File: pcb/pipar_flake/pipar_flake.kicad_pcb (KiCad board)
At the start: 2 copper layers, 74.1 x 55 mm, 22 parts, among them SW2 SW_Wuerth_450301014042, U2 nice_nano

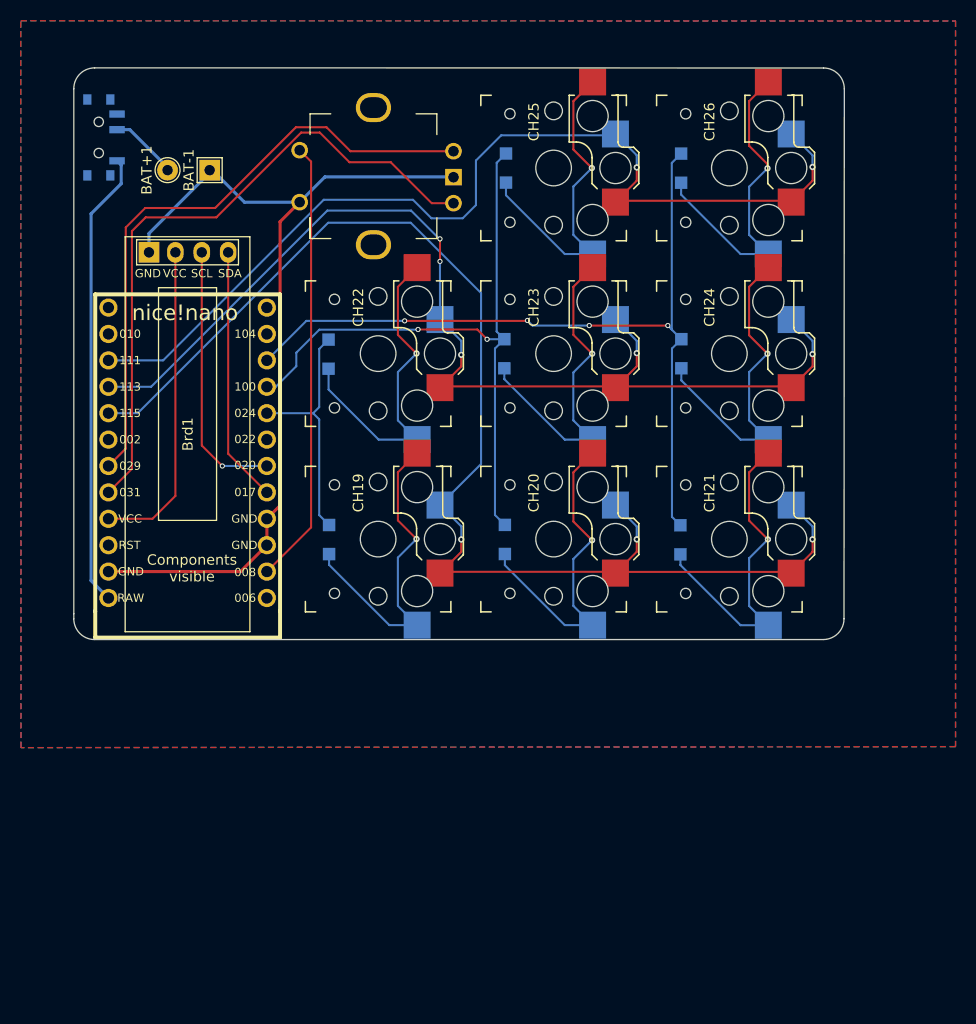
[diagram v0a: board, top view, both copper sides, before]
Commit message: Reworks Pipar Flake to add LEDs and a bigger place for battery
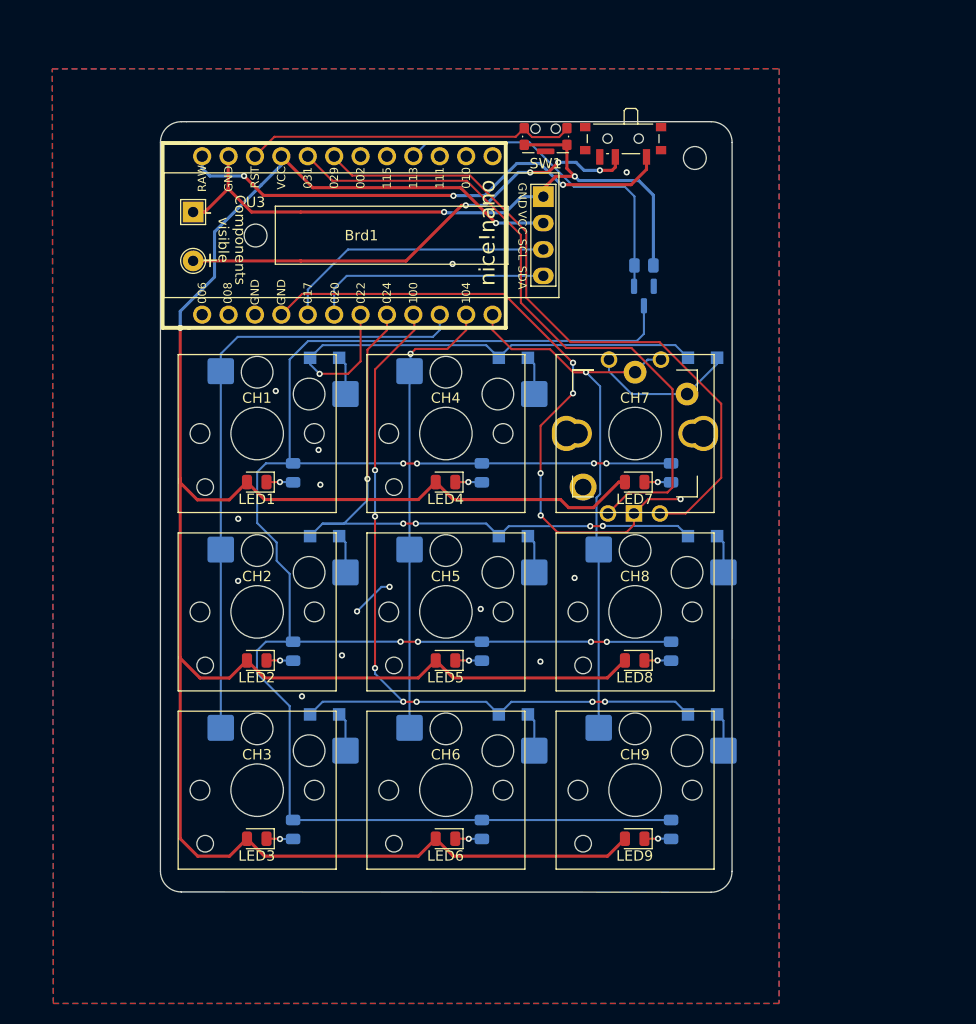
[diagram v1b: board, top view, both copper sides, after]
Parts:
- removed CH19, CH20, CH21, CH22, CH23, CH24, CH25, CH26: KSwitch, keyswitches:Kailh_socket_PG1350_reversible
- removed CH28: RotaryEncoder_Switch, Rotary_Encoder:RotaryEncoder_Bourns_Vertical_PEL11L-4xxxF-Sxxxx_1
- removed D19, D20, D21, D22, D23, D24, D25, D26: D, Diode_SMD:Nexperia_CFP3_SOD-123W
- added CH1: KSwitch, yes:SW_Hotswap_Kailh_Choc_V1V2_LED_1.00u, F.Cu at (32.8, 49.8)
- added CH10: RotaryEncoder_Switch, Rotary_Encoder:RotaryEncoder_Bourns_Vertical_PEL11L-4xxxF-Sxxxx_1, F.Cu at (69.1, 49.7)
- added CH2: KSwitch, yes:SW_Hotswap_Kailh_Choc_V1V2_LED_1.00u, F.Cu at (32.8, 66.9)
- added CH3: KSwitch, yes:SW_Hotswap_Kailh_Choc_V1V2_LED_1.00u, F.Cu at (32.8, 84.1)
- added CH4: KSwitch, yes:SW_Hotswap_Kailh_Choc_V1V2_LED_1.00u, F.Cu at (51.0, 49.8)
- added CH5: KSwitch, yes:SW_Hotswap_Kailh_Choc_V1V2_LED_1.00u, F.Cu at (51.0, 66.9)
- added CH6: KSwitch, yes:SW_Hotswap_Kailh_Choc_V1V2_LED_1.00u, F.Cu at (51.0, 84.1)
- added CH7: KSwitch, PCM_Switch_Keyboard_Kailh:SW_Kailh_Choc_V1V2_1.00u, F.Cu at (69.2, 49.8)
- added CH8: KSwitch, yes:SW_Hotswap_Kailh_Choc_V1V2_LED_1.00u, F.Cu at (69.2, 66.9)
- added CH9: KSwitch, yes:SW_Hotswap_Kailh_Choc_V1V2_LED_1.00u, F.Cu at (69.2, 84.1)
- added D1: D, Diode_SMD:Nexperia_CFP3_SOD-123W, B.Cu at (39.3, 42.5)
- added D2: D, Diode_SMD:Nexperia_CFP3_SOD-123W, B.Cu at (39.3, 59.7)
- added D3: D, Diode_SMD:Nexperia_CFP3_SOD-123W, B.Cu at (39.3, 76.8)
- added D4: D, Diode_SMD:Nexperia_CFP3_SOD-123W, B.Cu at (57.5, 42.5)
- added D5: D, Diode_SMD:Nexperia_CFP3_SOD-123W, B.Cu at (57.5, 59.7)
- added D6: D, Diode_SMD:Nexperia_CFP3_SOD-123W, B.Cu at (57.5, 76.8)
- added D7: D, Diode_SMD:Nexperia_CFP3_SOD-123W, B.Cu at (75.7, 42.5)
- added D8: D, Diode_SMD:Nexperia_CFP3_SOD-123W, B.Cu at (75.7, 59.6)
- added D9: D, Diode_SMD:Nexperia_CFP3_SOD-123W, B.Cu at (75.7, 76.8)
- added LED1: ~, LED_SMD:LED_0805_2012Metric, F.Cu at (32.8, 54.5)
- added LED2: ~, LED_SMD:LED_0805_2012Metric, F.Cu at (32.8, 71.6)
- added LED3: ~, LED_SMD:LED_0805_2012Metric, F.Cu at (32.8, 88.8)
- added LED4: ~, LED_SMD:LED_0805_2012Metric, F.Cu at (50.9, 54.5)
- added LED5: ~, LED_SMD:LED_0805_2012Metric, F.Cu at (50.9, 71.6)
- added LED6: ~, LED_SMD:LED_0805_2012Metric, F.Cu at (50.9, 88.8)
- added LED7: ~, LED_SMD:LED_0805_2012Metric, F.Cu at (69.1, 54.4)
- added LED8: ~, LED_SMD:LED_0805_2012Metric, F.Cu at (69.1, 71.6)
- added LED9: ~, LED_SMD:LED_0805_2012Metric, F.Cu at (69.1, 88.8)
- added Q1: AO3416 N-channel MOSFET, Package_TO_SOT_SMD:SOT-23, B.Cu at (70.0, 36.6)
- added R1: 100, Resistor_SMD:R_0805_2012Metric, B.Cu at (36.3, 53.6)
- added R10: 4.7k, Resistor_SMD:R_0805_2012Metric, B.Cu at (70.0, 33.6)
- added R2: 100, Resistor_SMD:R_0805_2012Metric, B.Cu at (36.3, 70.7)
- added R3: 100, Resistor_SMD:R_0805_2012Metric, B.Cu at (36.3, 87.9)
- added R4: 100, Resistor_SMD:R_0805_2012Metric, B.Cu at (54.4, 53.6)
- added R5: 100, Resistor_SMD:R_0805_2012Metric, B.Cu at (54.4, 70.7)
- added R6: 100, Resistor_SMD:R_0805_2012Metric, B.Cu at (54.4, 87.9)
- added R7: 100, Resistor_SMD:R_0805_2012Metric, B.Cu at (72.6, 53.6)
- added R8: 100, Resistor_SMD:R_0805_2012Metric, B.Cu at (72.6, 70.7)
- added R9: 100, Resistor_SMD:R_0805_2012Metric, B.Cu at (72.6, 87.9)
- added SW1: CK_KMS2xxG, Button_Switch_SMD:SW_SPST_CK_KMS2xxGP, F.Cu at (60.6, 21.2)
- added U1: ~, salt:Salt-smallest, F.Cu at (70.0, 32.0)
- added U3: ~, MountingHole:MountingHole_2.2mm_M2, F.Cu at (32.7, 30.7)
- added U4: nice_nano, nice-nano-kicad:nice_nano, F.Cu at (41.5, 30.7)
- SW2: moved to F.Cu
- U2: value nice_nano -> ~; footprint nice-nano-kicad:nice_nano -> MountingHole:MountingHole_2.2mm_M2
- moved U2 56.4 mm to (74.9, 23.3), turned to 0 degrees
- moved SW2 50.1 mm to (68.0, 21.7), turned to 180 degrees
- moved Brd1 25.4 mm to (42.8, 30.7), turned to -90 degrees
- moved BAT+1 9.07 mm to (26.6, 33.2), turned to 0 degrees
- moved BAT-1 4.33 mm to (26.6, 28.5), turned to 0 degrees
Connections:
- Brd1 pad 2: Net-(Brd1-VCC) -> +3.3V
- Brd1 pad 3: Net-(Brd1-SCL) -> SCL
- Brd1 pad 4: Net-(Brd1-SDA) -> SDA
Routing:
- net +3.3V: track 0.00 -> 239.6 mm, vias 0 -> 2
- net LEDOut: track 0.00 -> 200.2 mm, vias 0 -> 8
- net Net-(U2-P1.15): track 127.6 -> 0.00 mm, vias 3 -> 0
- net Net-(U2-P1.13): track 106.6 -> 0.00 mm, vias 5 -> 0
- net Net-(U2-P1.11): track 95.3 -> 0.00 mm, vias 2 -> 0
- net ROW2: track 0.00 -> 78.4 mm, vias 0 -> 7
- net Net-(D21-K): track 78.1 -> 0.00 mm, vias 4 -> 0
- net Net-(U4-AIN5/P0.29): track 0.00 -> 65.4 mm
- net Net-(U4-AIN7/P0.31): track 0.00 -> 64.9 mm
- net Net-(U2-AIN7/P0.31): track 63.8 -> 0.00 mm
- net Net-(D20-K): track 63.5 -> 0.00 mm, vias 2 -> 0
- net ROW1: track 0.00 -> 62.1 mm, vias 0 -> 5
- net Net-(U2-AIN5/P0.29): track 60.1 -> 0.00 mm
- net COL0: track 0.00 -> 59.5 mm
- net COL2: track 0.00 -> 54.9 mm, vias 0 -> 1
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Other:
- board size 74.1 x 55 mm -> 55 x 74.1 mm
- board text added: "+"
- board text added: "-"

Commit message: slightly change the cut to be more straight
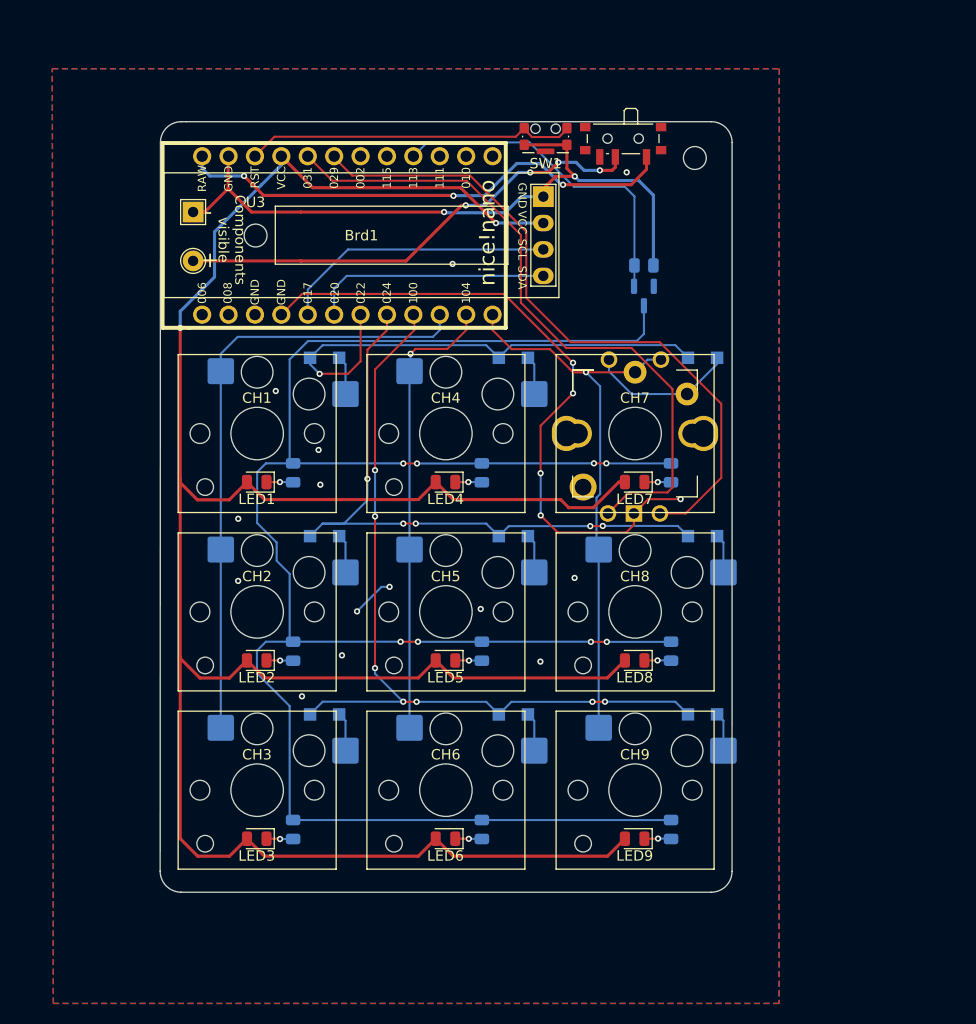
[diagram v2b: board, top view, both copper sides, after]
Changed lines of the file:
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@@
 	)
 	(gr_arc
-		(start 25.503837 93.880692)
-		(mid 24.090391 93.294468)
-		(end 23.504933 91.880693)
+		(start 25.503829 93.908505)
+		(mid 24.070704 93.314136)
+		(end 23.477095 91.880696)
 		(stroke
 			(width 0.05)
@@
 	)
 	(gr_line
-		(start 23.504933 91.880693)
+		(start 23.477095 91.880696)
 		(end 23.504926 21.779597)
 		(stroke
@@
 	(gr_line
 		(start 76.494113 93.908505)
-		(end 25.503837 93.880692)
+		(end 25.503829 93.908505)
 		(stroke
 			(width 0.05)
